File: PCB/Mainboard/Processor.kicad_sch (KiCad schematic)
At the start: 1 part, among them U76 80486SX

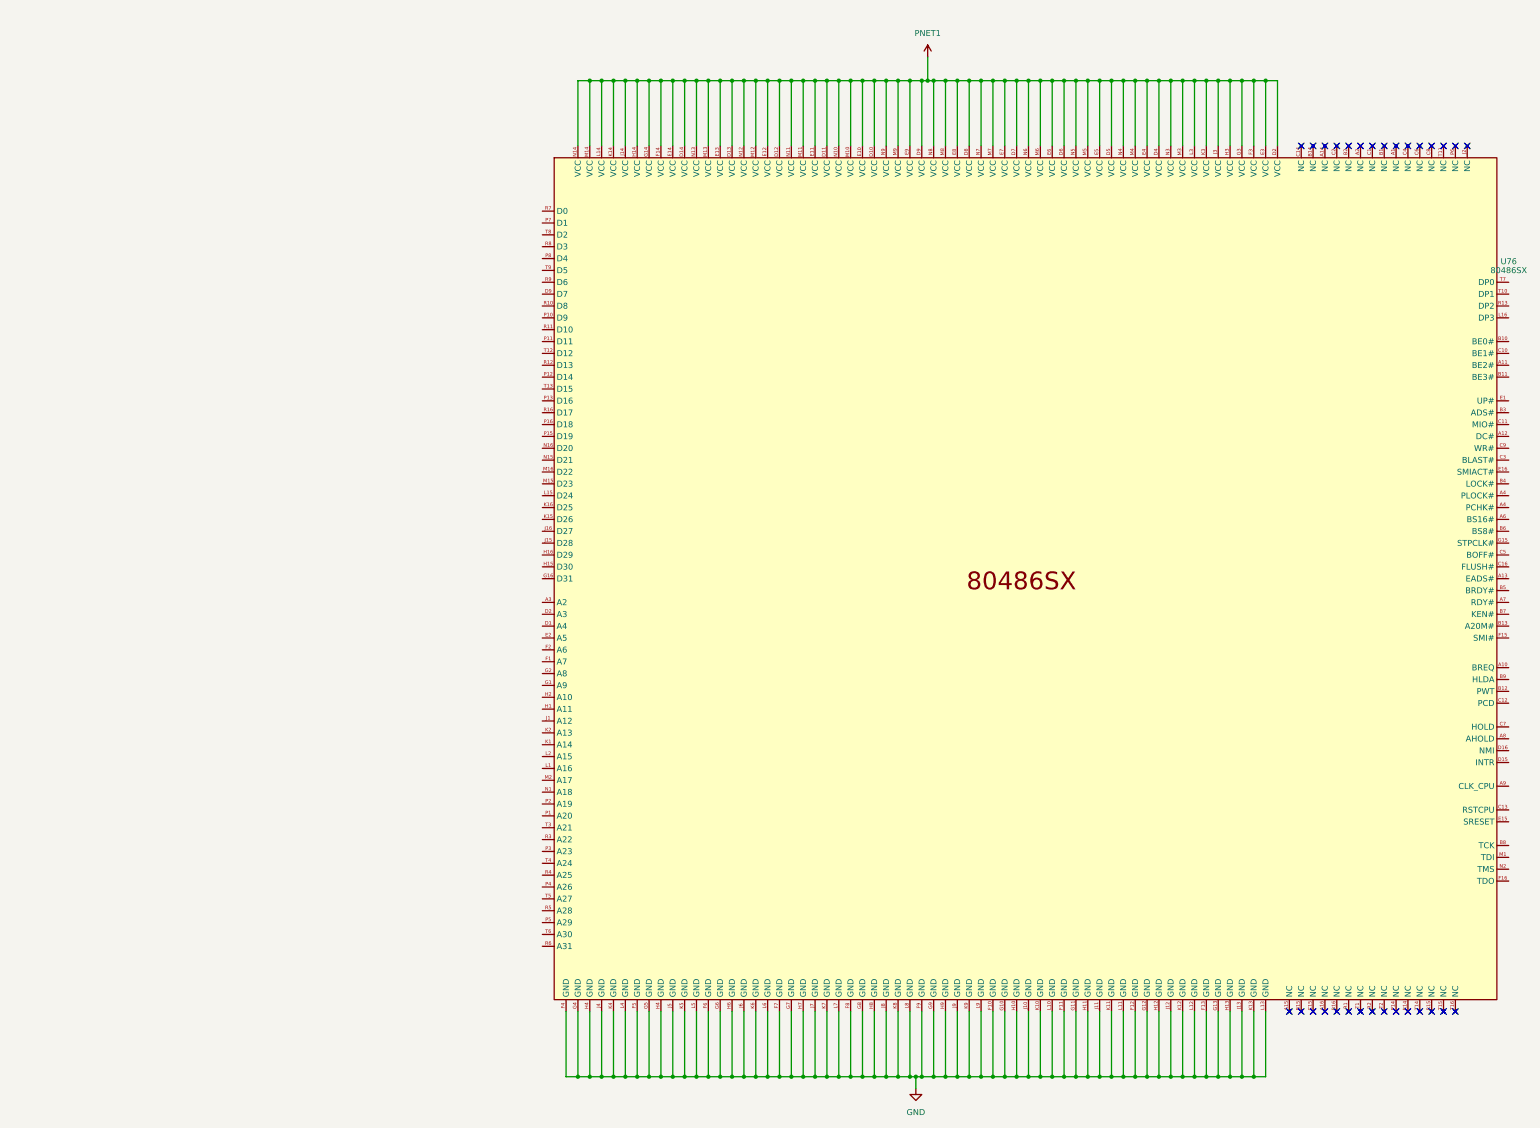
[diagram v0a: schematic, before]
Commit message: Add files via upload
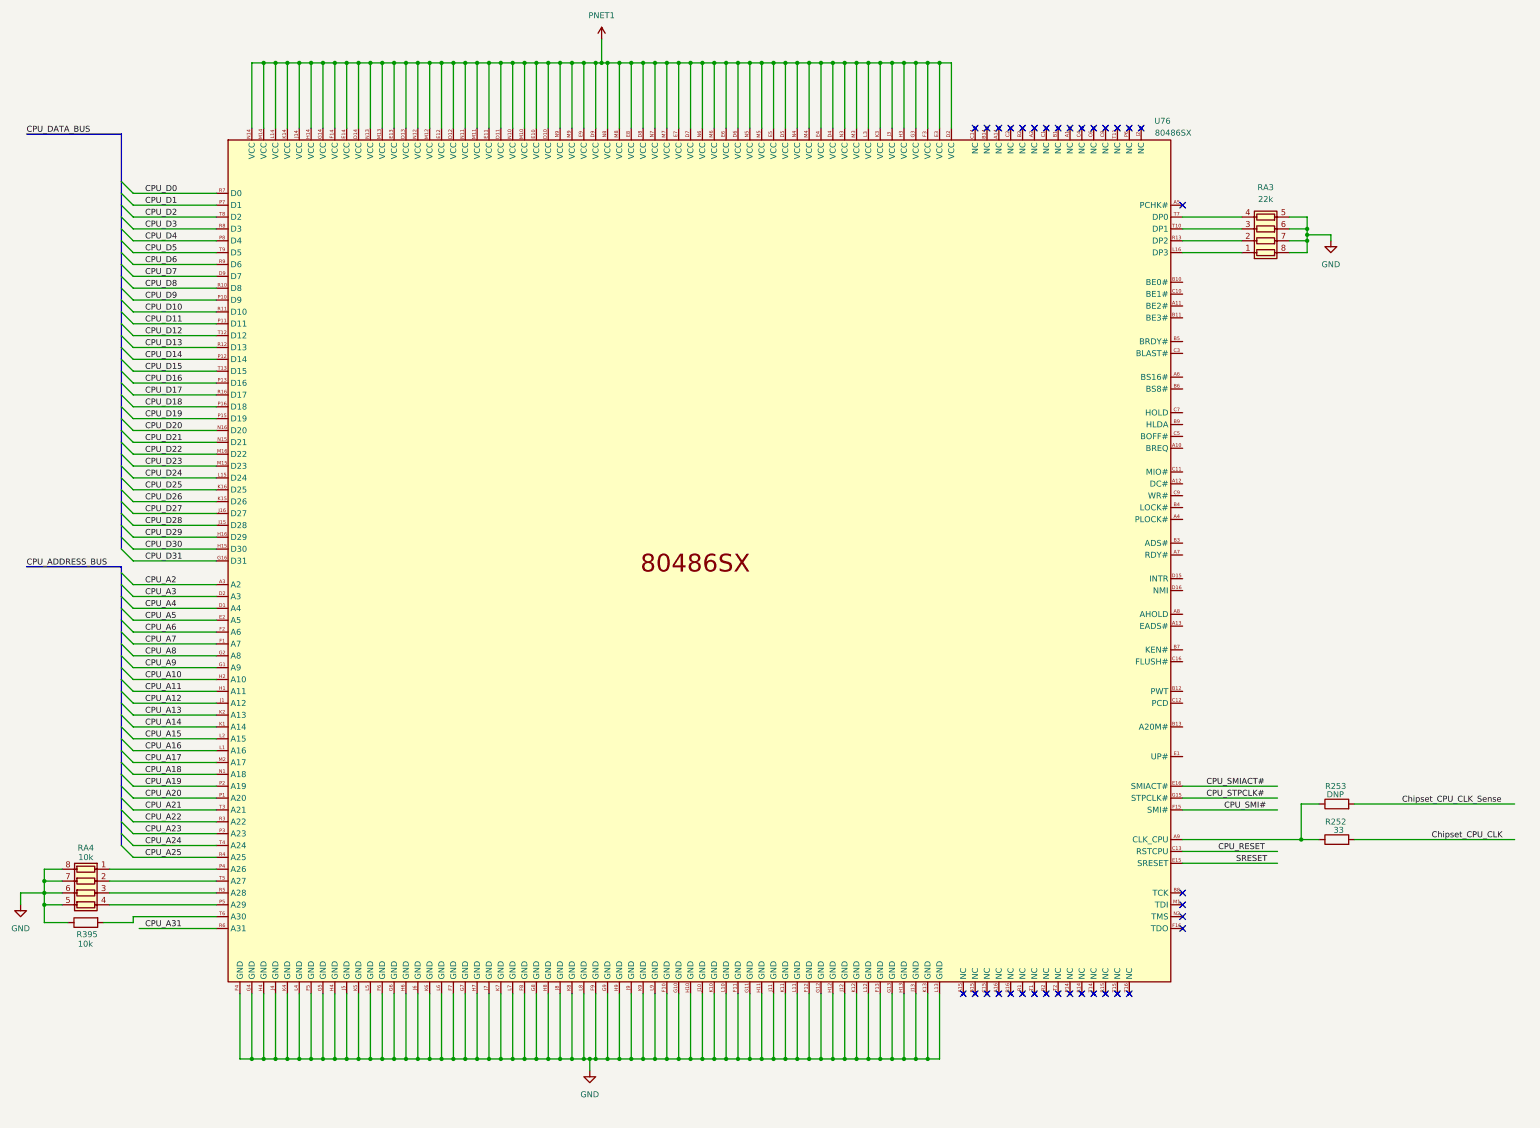
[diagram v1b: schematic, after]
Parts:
- added R252: 33, symbol Device:R
- added R253: DNP, symbol Device:R
- added R395: 10k, symbol Device:R
- added RA3: 22k, symbol Device:R_Pack04
- added RA4: 10k, symbol Device:R_Pack04
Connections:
- net GND: now also R395.1, RA3.5 (R4.2), RA3.6 (R3.2), RA3.7 (R2.2), RA3.8 (R1.2), RA4.5 (R4.2), RA4.6 (R3.2), RA4.7 (R2.2), RA4.8 (R1.2)
- net CPU_A2: now reaches U76.A3 (A2)
- net at U76.A9 (CLK_CPU): now also R252.1, R253.1
- net CPU_RESET: now reaches U76.C13 (RSTCPU)
- net CPU_A4: now reaches U76.D1 (A4)
- net SRESET: now reaches U76.E15 (SRESET)
- net CPU_SMIACT#: now reaches U76.E16 (SMIACT#)
- net CPU_A5: now reaches U76.E2 (A5)
- net CPU_A7: now reaches U76.F1 (A7)
- net CPU_SMI#: now reaches U76.F15 (SMI#)
- net CPU_A6: now reaches U76.F2 (A6)
- net CPU_A9: now reaches U76.G1 (A9)
- net CPU_STPCLK#: now reaches U76.G15 (STPCLK#)
- net CPU_D31: now reaches U76.G16 (D31)
- net CPU_A8: now reaches U76.G2 (A8)
- net CPU_A11: now reaches U76.H1 (A11)
- net CPU_D30: now reaches U76.H15 (D30)
- net CPU_D29: now reaches U76.H16 (D29)
- net CPU_A10: now reaches U76.H2 (A10)
- net CPU_A12: now reaches U76.J1 (A12)
- net CPU_D28: now reaches U76.J15 (D28)
- net CPU_D27: now reaches U76.J16 (D27)
- net CPU_A14: now reaches U76.K1 (A14)
- net CPU_D26: now reaches U76.K15 (D26)
- net CPU_D25: now reaches U76.K16 (D25)
- net CPU_A13: now reaches U76.K2 (A13)
- net CPU_A16: now reaches U76.L1 (A16)
- net CPU_D24: now reaches U76.L15 (D24)
- net at U76.L16 (DP3): now also RA3.1 (R1.1)
- net CPU_A15: now reaches U76.L2 (A15)
- net CPU_D23: now reaches U76.M15 (D23)
- net CPU_D22: now reaches U76.M16 (D22)
- net CPU_A17: now reaches U76.M2 (A17)
- net CPU_A18: now reaches U76.N1 (A18)
- net CPU_D21: now reaches U76.N15 (D21)
- net CPU_D20: now reaches U76.N16 (D20)
- net CPU_A20: now reaches U76.P1 (A20)
- net CPU_D9: now reaches U76.P10 (D9)
- net CPU_D11: now reaches U76.P11 (D11)
- net CPU_D14: now reaches U76.P12 (D14)
- net CPU_D16: now reaches U76.P13 (D16)
- net CPU_D19: now reaches U76.P15 (D19)
- net CPU_D18: now reaches U76.P16 (D18)
- net CPU_A19: now reaches U76.P2 (A19)
- net CPU_A23: now reaches U76.P3 (A23)
- net at U76.P4 (A26): now also RA4.1 (R1.1)
- net at U76.P5 (A29): now also RA4.4 (R4.1)
- net CPU_D1: now reaches U76.P7 (D1)
- net CPU_D4: now reaches U76.P8 (D4)
- net CPU_D8: now reaches U76.R10 (D8)
- net CPU_D10: now reaches U76.R11 (D10)
- net CPU_D13: now reaches U76.R12 (D13)
- net at U76.R13 (DP2): now also RA3.2 (R2.1)
- net CPU_D17: now reaches U76.R16 (D17)
- net CPU_A22: now reaches U76.R3 (A22)
- net CPU_A25: now reaches U76.R4 (A25)
- net at U76.R5 (A28): now also RA4.3 (R3.1)
- net CPU_A31: now reaches U76.R6 (A31)
- net CPU_D0: now reaches U76.R7 (D0)
- net CPU_D3: now reaches U76.R8 (D3)
- net CPU_D6: now reaches U76.R9 (D6)
- net at U76.T10 (DP1): now also RA3.3 (R3.1)
- net CPU_D12: now reaches U76.T12 (D12)
- net CPU_D15: now reaches U76.T13 (D15)
- net CPU_A21: now reaches U76.T3 (A21)
- net CPU_A24: now reaches U76.T4 (A24)
- net at U76.T5 (A27): now also RA4.2 (R2.1)
- net at U76.T6 (A30): now also R395.2
- net at U76.T7 (DP0): now also RA3.4 (R4.1)
- net CPU_D2: now reaches U76.T8 (D2)
- net CPU_D5: now reaches U76.T9 (D5)
- new net CPU_A3: U76.D2 (VCC)
- new net CPU_D7: U76.D9 (VCC)
- new net Chipset_CPU_CLK: R252.2
- new net Chipset_CPU_CLK_Sense: R253.2
- no-connect marks 30 -> 35
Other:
- moved on the sheet: U76
